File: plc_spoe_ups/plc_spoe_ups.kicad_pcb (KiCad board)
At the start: 4 copper layers, 1.3 x 1.3 mm, 2 parts

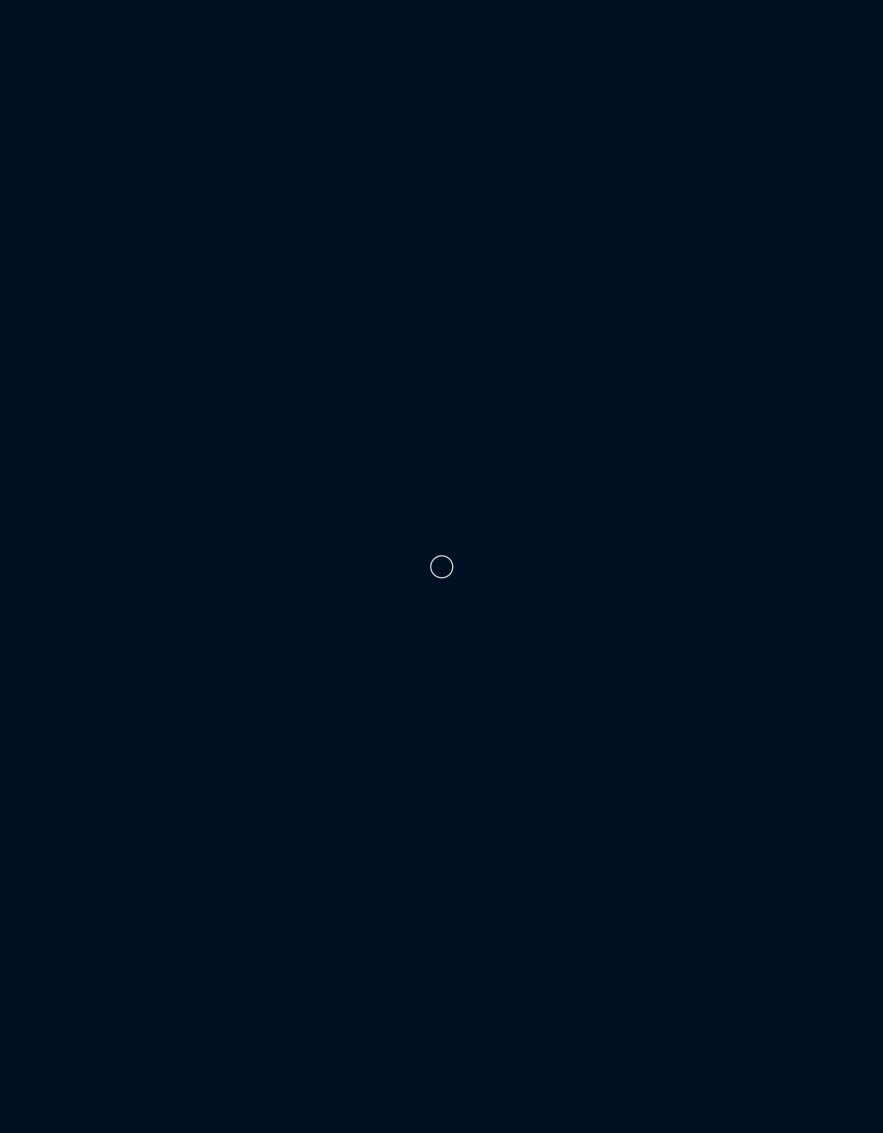
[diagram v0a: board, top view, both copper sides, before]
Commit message: refactor: Update KiCad PCB file
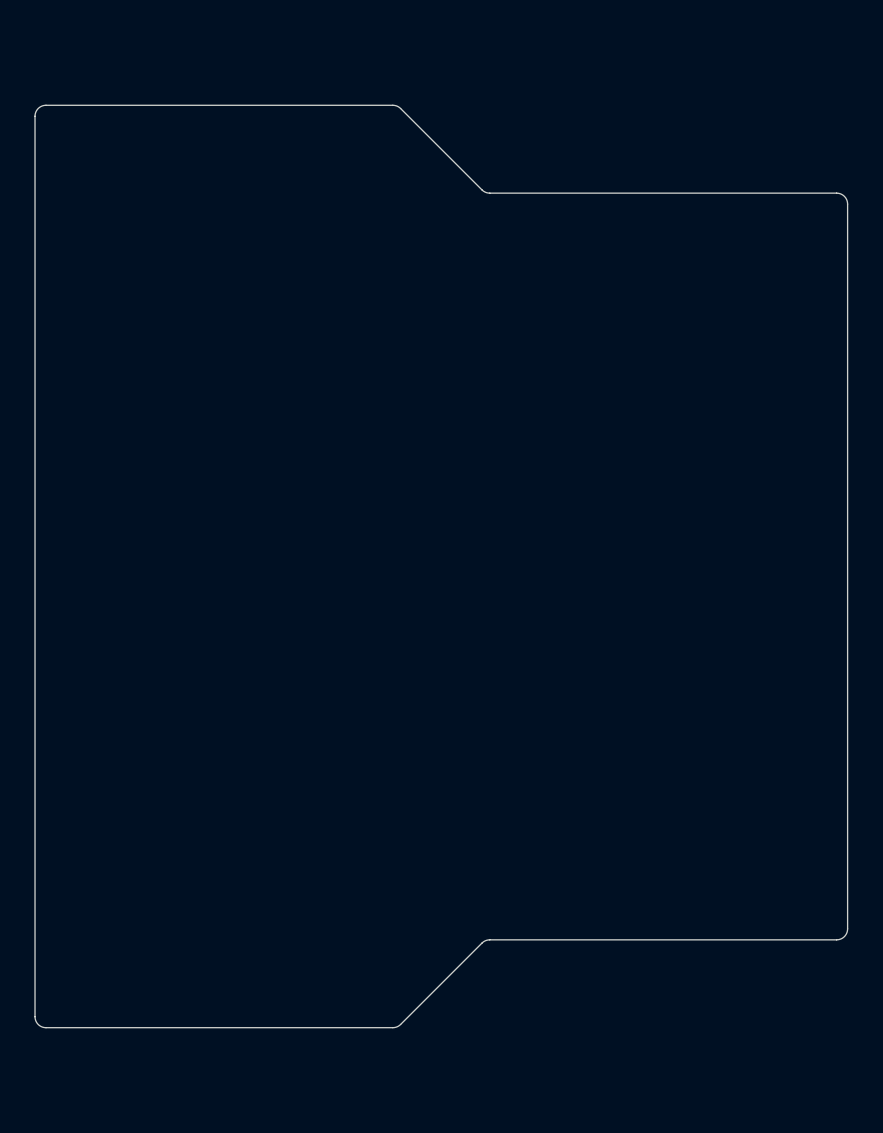
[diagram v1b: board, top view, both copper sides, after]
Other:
- board size 1.3 x 1.3 mm -> 47 x 53.3 mm
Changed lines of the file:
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@@
 	(footprint "modules_footprints:supercap_bank"
 		(layer "F.Cu")
-		(at 121.7676 93.18498)
+		(at 121.7676 93.1672)
 		(property "Reference" "A2"
 			(at 0 0 0)
@@
 	(footprint "modules_footprints:minimal_ltc3350"
 		(layer "F.Cu")
-		(at 130.896473 93.185256)
+		(at 130.8608 93.1672)
 		(property "Reference" "A1"
 			(at 0 -0.5 0)
@@
 		)
 	)
-	(gr_circle
-		(center 130.8862 93.185256)
-		(end 131.5212 93.185256)
-		(stroke
-			(width 0.05)
-			(type default)
-		)
-		(fill no)
-		(layer "Edge.Cuts")
-	)
+	(gr_arc
+		(start 107.3658 67.1322)
+		(mid 107.551787 66.683187)
+		(end 108.0008 66.4972)
+		(stroke
+			(width 0.05)
+			(type default)
+		)
+		(layer "Edge.Cuts")
+	)
+	(gr_line
+		(start 128.506787 119.651213)
+		(end 133.214813 114.943187)
+		(stroke
+			(width 0.05)
+			(type default)
+		)
+		(layer "Edge.Cuts")
+	)
+	(gr_arc
+		(start 153.7208 71.5772)
+		(mid 154.169813 71.763187)
+		(end 154.3558 72.2122)
+		(stroke
+			(width 0.05)
+			(type default)
+		)
+		(layer "Edge.Cuts")
+	)
+	(gr_arc
+		(start 128.057774 66.4972)
+		(mid 128.300783 66.545528)
+		(end 128.506787 66.683187)
+		(stroke
+			(width 0.05)
+			(type default)
+		)
+		(layer "Edge.Cuts")
+	)
+	(gr_line
+		(start 108.0008 119.8372)
+		(end 128.057774 119.8372)
+		(stroke
+			(width 0.05)
+			(type default)
+		)
+		(layer "Edge.Cuts")
+	)
+	(gr_line
+		(start 154.3558 114.1222)
+		(end 154.3558 72.2122)
+		(stroke
+			(width 0.05)
+			(type default)
+		)
+		(layer "Edge.Cuts")
+	)
+	(gr_line
+		(start 107.3658 67.1322)
+		(end 107.3658 119.2022)
+		(stroke
+			(width 0.05)
+			(type default)
+		)
+		(layer "Edge.Cuts")
+	)
+	(gr_arc
+		(start 133.214813 114.943187)
+		(mid 133.420823 114.805545)
+		(end 133.663826 114.7572)
+		(stroke
+			(width 0.05)
+			(type default)
+		)
+		(layer "Edge.Cuts")
+	)
+	(gr_arc
+		(start 133.663826 71.5772)
+		(mid 133.420822 71.528864)
+		(end 133.214813 71.391213)
+		(stroke
+			(width 0.05)
+			(type default)
+		)
+		(layer "Edge.Cuts")
+	)
+	(gr_arc
+		(start 108.0008 119.8372)
+		(mid 107.551787 119.651213)
+		(end 107.3658 119.2022)
+		(stroke
+			(width 0.05)
+			(type default)
+		)
+		(layer "Edge.Cuts")
+	)
+	(gr_line
+		(start 128.057774 66.4972)
+		(end 108.0008 66.4972)
+		(stroke
+			(width 0.05)
+			(type default)
+		)
+		(layer "Edge.Cuts")
+	)
+	(gr_line
+		(start 133.663826 114.7572)
+		(end 153.7208 114.7572)
+		(stroke
+			(width 0.05)
+			(type default)
+		)
+		(layer "Edge.Cuts")
+	)
+	(gr_line
+		(start 153.7208 71.5772)
+		(end 133.663826 71.5772)
+		(stroke
+			(width 0.05)
+			(type default)
+		)
+		(layer "Edge.Cuts")
+	)
+	(gr_arc
+		(start 154.3558 114.1222)
+		(mid 154.169813 114.571213)
+		(end 153.7208 114.7572)
+		(stroke
+			(width 0.05)
+			(type default)
+		)
+		(layer "Edge.Cuts")
+	)
+	(gr_line
+		(start 133.214813 71.391213)
+		(end 128.506787 66.683187)
+		(stroke
+			(width 0.05)
+			(type default)
+		)
+		(layer "Edge.Cuts")
+	)
+	(gr_arc
+		(start 128.506787 119.651213)
+		(mid 128.300777 119.788855)
+		(end 128.057774 119.8372)
+		(stroke
+			(width 0.05)
+			(type default)
+		)
+		(layer "Edge.Cuts")
+	)

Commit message: Update KiCAD Symbols Generator and PCB file
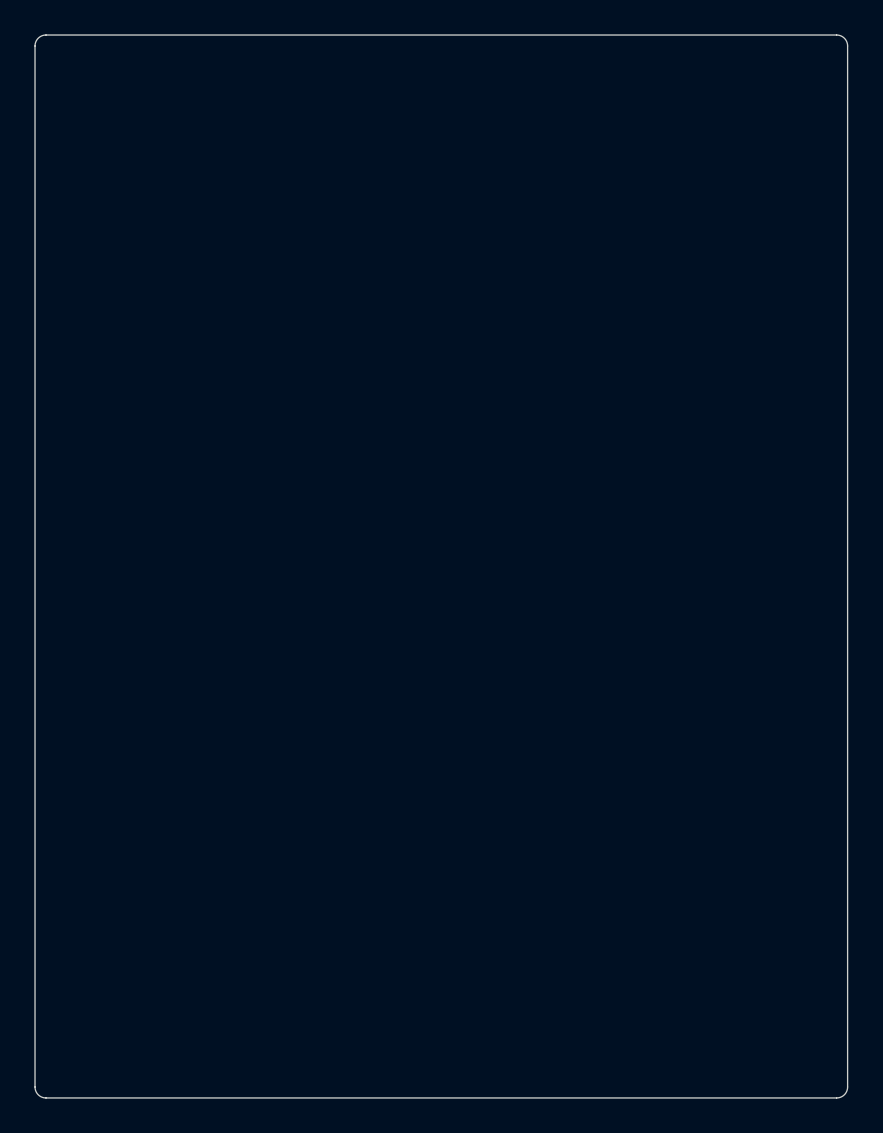
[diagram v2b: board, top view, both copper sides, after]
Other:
- board size 47 x 53.3 mm -> 47 x 61.5 mm
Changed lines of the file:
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@@
 		(sheetfile "plc_spoe_ups.kicad_sch")
 		(fp_line
-			(start -23.495 26.035)
-			(end -23.495 -26.035)
+			(start -23.495 30.099)
+			(end -23.495 -30.099)
 			(stroke
 				(width 0.05)
@@
 		)
 		(fp_line
-			(start -22.86 -26.67)
-			(end -2.803 -26.67)
+			(start -22.86 -30.734)
+			(end 22.86 -30.734)
 			(stroke
 				(width 0.05)
@@
 		)
 		(fp_line
-			(start -2.803026 26.67)
-			(end -22.86 26.67)
+			(start 22.86 30.734)
+			(end -22.86 30.734)
 			(stroke
 				(width 0.05)
@@
 		)
 		(fp_line
-			(start 2.354013 -21.775987)
-			(end -2.354013 -26.484013)
-			(stroke
-				(width 0.05)
-				(type default)
-			)
-			(layer "Cmts.User")
-		)
-		(fp_line
-			(start 2.354013 21.775987)
-			(end -2.354013 26.484013)
-			(stroke
-				(width 0.05)
-				(type default)
-			)
-			(layer "Cmts.User")
-		)
-		(fp_line
-			(start 22.86 -21.59)
-			(end 2.803026 -21.59)
-			(stroke
-				(width 0.05)
-				(type default)
-			)
-			(layer "Cmts.User")
-		)
-		(fp_line
-			(start 22.86 21.59)
-			(end 2.803026 21.59)
-			(stroke
-				(width 0.05)
-				(type default)
-			)
-			(layer "Cmts.User")
-		)
-		(fp_line
-			(start 23.495 -20.955)
-			(end 23.495 20.955)
+			(start 23.495 -30.099)
+			(end 23.495 30.099)
 			(stroke
 				(width 0.05)
@@
 		)
 		(fp_arc
-			(start -23.495 -26.035)
-			(mid -23.309013 -26.484013)
-			(end -22.86 -26.67)
+			(start -23.495 -30.099)
+			(mid -23.309013 -30.548013)
+			(end -22.86 -30.734)
 			(stroke
 				(width 0.05)
@@
 		)
 		(fp_arc
-			(start -22.86 26.67)
-			(mid -23.309013 26.484013)
-			(end -23.495 26.035)
+			(start -22.86 30.734)
+			(mid -23.309013 30.548013)
+			(end -23.495 30.099)
 			(stroke
 				(width 0.05)
@@
 		)
 		(fp_arc
-			(start -2.803026 -26.67)
-			(mid -2.560017 -26.621672)
-			(end -2.354013 -26.484013)
+			(start 22.86 -30.734)
+			(mid 23.309013 -30.548013)
+			(end 23.495 -30.099)
 			(stroke
 				(width 0.05)
@@
 		)
 		(fp_arc
-			(start -2.354013 26.484013)
-			(mid -2.560023 26.621655)
-			(end -2.803026 26.67)
-			(stroke
-				(width 0.05)
-				(type default)
-			)
-			(layer "Cmts.User")
-		)
-		(fp_arc
-			(start 2.354013 21.775987)
-			(mid 2.560023 21.638345)
-			(end 2.803026 21.59)
-			(stroke
-				(width 0.05)
-				(type default)
-			)
-			(layer "Cmts.User")
-		)
-		(fp_arc
-			(start 2.803026 -21.59)
-			(mid 2.560022 -21.638336)
-			(end 2.354013 -21.775987)
-			(stroke
-				(width 0.05)
-				(type default)
-			)
-			(layer "Cmts.User")
-		)
-		(fp_arc
-			(start 22.86 -21.59)
-			(mid 23.309013 -21.404013)
-			(end 23.495 -20.955)
-			(stroke
-				(width 0.05)
-				(type default)
-			)
-			(layer "Cmts.User")
-		)
-		(fp_arc
-			(start 23.495 20.955)
-			(mid 23.309013 21.404013)
-			(end 22.86 21.59)
+			(start 23.495 30.099)
+			(mid 23.309013 30.548013)
+			(end 22.86 30.734)
 			(stroke
 				(width 0.05)
@@
 		)
 	)
+	(gr_line
+		(start 153.7208 123.9012)
+		(end 108.0008 123.9012)
+		(stroke
+			(width 0.05)
+			(type default)
+		)
+		(layer "Edge.Cuts")
+	)
 	(gr_arc
-		(start 107.3658 67.1322)
-		(mid 107.551787 66.683187)
-		(end 108.0008 66.4972)
+		(start 107.365799 63.068201)
+		(mid 107.551786 62.619188)
+		(end 108.000799 62.433201)
+		(stroke
+			(width 0.05)
+			(type default)
+		)
+		(layer "Edge.Cuts")
+	)
+	(gr_arc
+		(start 153.720801 62.433201)
+		(mid 154.169814 62.619188)
+		(end 154.355801 63.068201)
 		(stroke
 			(width 0.05)
@@
 	)
 	(gr_line
-		(start 128.506787 119.651213)
-		(end 133.214813 114.943187)
+		(start 154.3558 123.2662)
+		(end 154.3558 63.068201)
+		(stroke
+			(width 0.05)
+			(type default)
+		)
+		(layer "Edge.Cuts")
+	)
+	(gr_line
+		(start 107.3658 63.068201)
+		(end 107.3658 123.2662)
 		(stroke
 			(width 0.05)
@@
 	)
 	(gr_arc
-		(start 153.7208 71.5772)
-		(mid 154.169813 71.763187)
-		(end 154.3558 72.2122)
+		(start 108.000799 123.9012)
+		(mid 107.551786 123.715213)
+		(end 107.365799 123.2662)
+		(stroke
+			(width 0.05)
+			(type default)
+		)
+		(layer "Edge.Cuts")
+	)
+	(gr_line
+		(start 153.7208 62.433201)
+		(end 108.000799 62.433201)
 		(stroke
 			(width 0.05)
@@
 	)
 	(gr_arc
-		(start 128.057774 66.4972)
-		(mid 128.300783 66.545528)
-		(end 128.506787 66.683187)
+		(start 154.3558 123.2662)
+		(mid 154.169813 123.715213)
+		(end 153.7208 123.9012)
 		(stroke
 			(width 0.05)
-			(type default)
-		)
-		(layer "Edge.Cuts")
-	)
-	(gr_line
-		(start 108.0008 119.8372)
-		(end 128.057774 119.8372)
-		(stroke
-			(width 0.05)
-			(type default)
-		)
-		(layer "Edge.Cuts")
-	)
-	(gr_line
-		(start 154.3558 114.1222)
-		(end 154.3558 72.2122)
-		(stroke
-			(width 0.05)
-			(type default)
-		)
-		(layer "Edge.Cuts")
-	)
-	(gr_line
-		(start 107.3658 67.1322)
-		(end 107.3658 119.2022)
-		(stroke
-			(width 0.05)
-			(type default)
-		)
-		(layer "Edge.Cuts")
-	)
-	(gr_arc
-		(start 133.214813 114.943187)
-		(mid 133.420823 114.805545)
-		(end 133.663826 114.7572)
-		(stroke
-			(width 0.05)
-			(type default)
-		)
-		(layer "Edge.Cuts")
-	)
-	(gr_arc
-		(start 133.663826 71.5772)
-		(mid 133.420822 71.528864)
-		(end 133.214813 71.391213)
-		(stroke
-			(width 0.05)
-			(type default)
-		)
-		(layer "Edge.Cuts")
-	)
-	(gr_arc
-		(start 108.0008 119.8372)
-		(mid 107.551787 119.651213)
-		(end 107.3658 119.2022)
-		(stroke
-			(width 0.05)
-			(type default)
-		)
-		(layer "Edge.Cuts")
-	)
-	(gr_line
-		(start 128.057774 66.4972)
-		(end 108.0008 66.4972)
-		(stroke
-			(width 0.05)
-			(type default)
-		)
-		(layer "Edge.Cuts")
-	)
-	(gr_line
-		(start 133.663826 114.7572)
-		(end 153.7208 114.7572)
-		(stroke
-			(width 0.05)
-			(type default)
-		)
-		(layer "Edge.Cuts")
-	)
-	(gr_line
-		(start 153.7208 71.5772)
-		(end 133.663826 71.5772)
-		(stroke
-			(width 0.05)
-			(type default)
-		)
-		(layer "Edge.Cuts")
-	)
-	(gr_arc
-		(start 154.3558 114.1222)
-		(mid 154.169813 114.571213)
-		(end 153.7208 114.7572)
-		(stroke
-			(width 0.05)
-			(type default)
-		)
-		(layer "Edge.Cuts")
-	)
-	(gr_line
-		(start 133.214813 71.391213)
-		(end 128.506787 66.683187)
-		(stroke
-			(width 0.05)
-			(type default)
-		)
-		(layer "Edge.Cuts")
-	)
-	(gr_arc
-		(start 128.506787 119.651213)
-		(mid 128.300777 119.788855)
-		(end 128.057774 119.8372)
-		(stroke
-			(width 0.05)
